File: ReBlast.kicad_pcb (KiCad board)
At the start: 2 copper layers, 50.7 x 64.9 mm, 23 parts, among them J1 MOS_8580_Socket, U1 74HC20, U2 74HC139, U3 ZN428E-8, U4 TLC272, U5 MOS_8580, U6 ADC0804

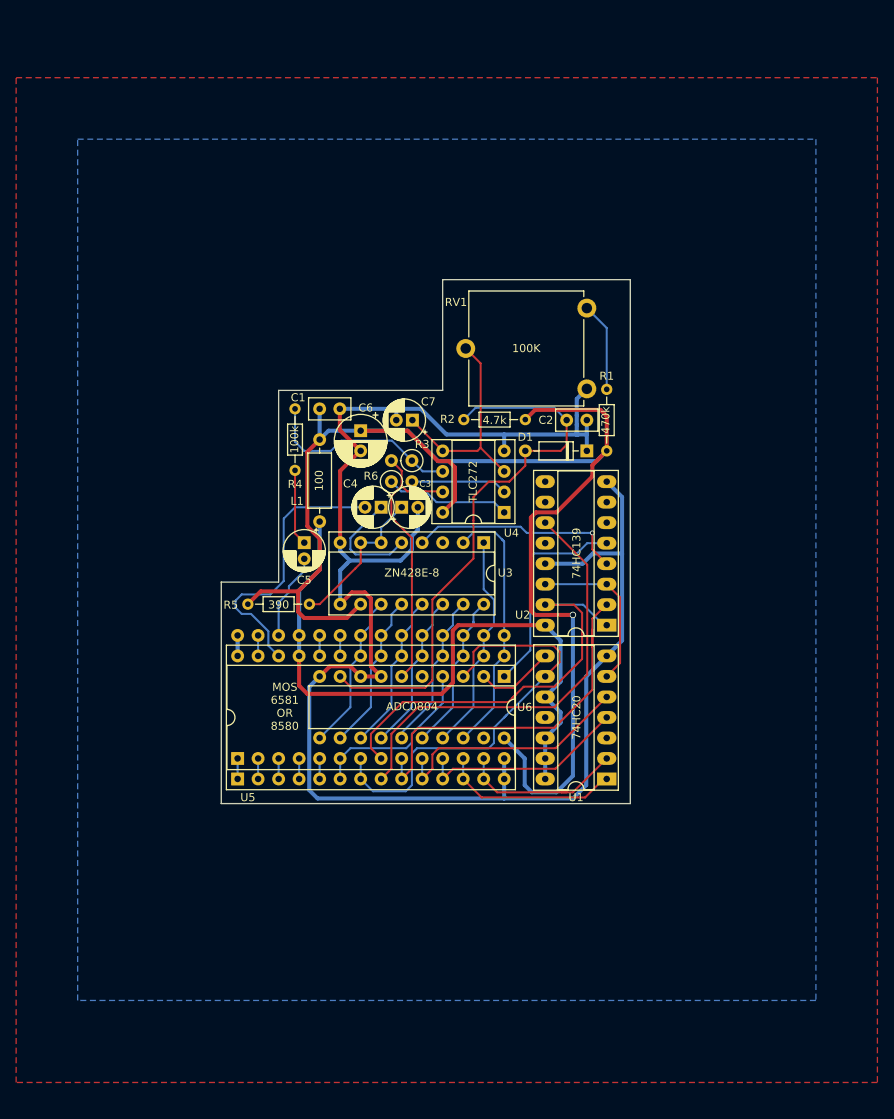
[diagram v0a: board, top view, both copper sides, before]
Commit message: Almost there...
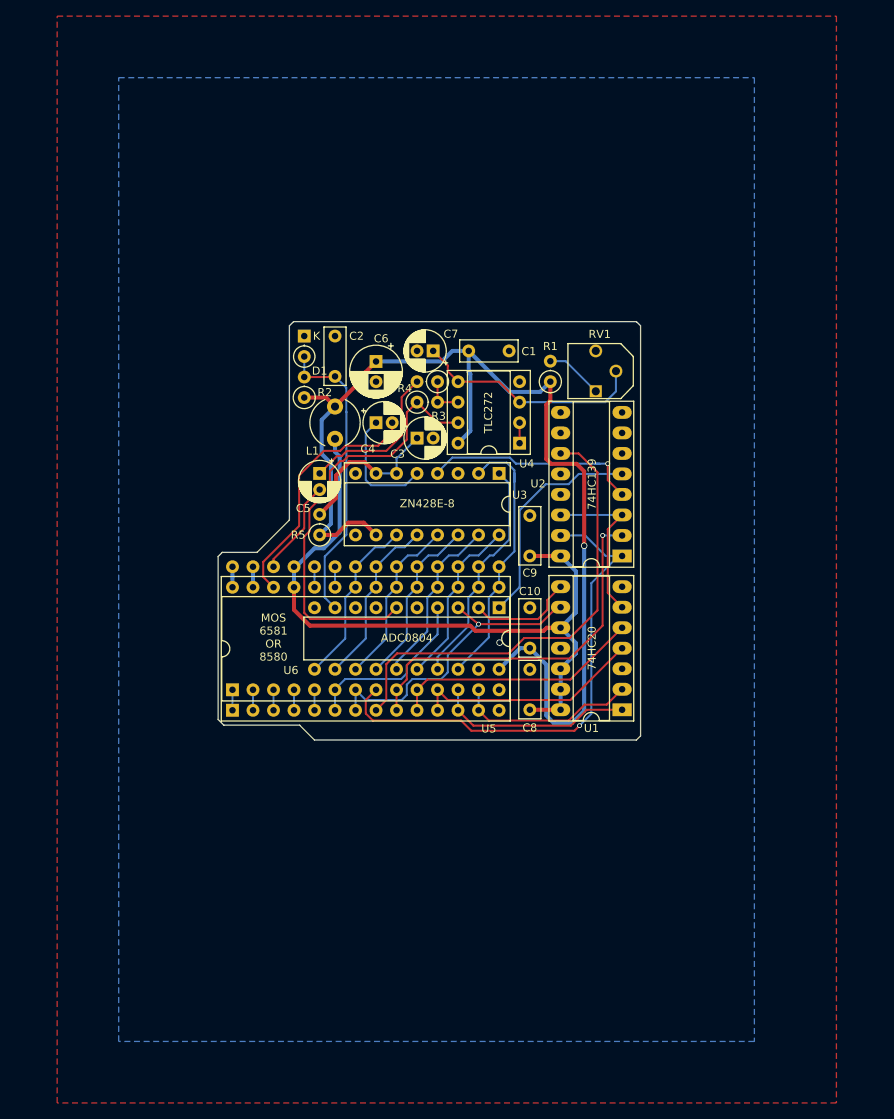
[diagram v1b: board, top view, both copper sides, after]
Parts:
- removed R6: 330k, Resistor_THT:R_Axial_DIN0207_L6.3mm_D2.5mm_P2.54mm_Vertical
- added C10: 100n, Capacitor_THT:C_Disc_D7.0mm_W2.5mm_P5.00mm, F.Cu at (165.2, 108.8)
- added C8: 100n, Capacitor_THT:C_Disc_D7.0mm_W2.5mm_P5.00mm, F.Cu at (165.2, 116.4)
- added C9: 100n, Capacitor_THT:C_Disc_D7.0mm_W2.5mm_P5.00mm, F.Cu at (165.2, 97.3)
- C1, C2: footprint Capacitor_THT:C_Disc_D5.0mm_W2.5mm_P2.50mm -> Capacitor_THT:C_Disc_D7.0mm_W2.5mm_P5.00mm
- D1: footprint Diode_THT:D_DO-35_SOD27_P7.62mm_Horizontal -> Diode_THT:D_DO-35_SOD27_P2.54mm_Vertical_KathodeUp
- L1: footprint Inductor_THT:L_Axial_L6.6mm_D2.7mm_P10.16mm_Horizontal_Vishay_IM-2 -> Inductor_THT:L_Radial_D6.0mm_P4.00mm
- R1, R2, R4, R5: footprint Resistor_THT:R_Axial_DIN0204_L3.6mm_D1.6mm_P7.62mm_Horizontal -> Resistor_THT:R_Axial_DIN0207_L6.3mm_D2.5mm_P2.54mm_Vertical
- RV1: footprint Potentiometer_THT:Potentiometer_ACP_CA14V-15_Vertical -> ReBlast:Pot_Bourns_3306P
- moved D1 37.8 mm to (137.3, 70.1), turned to 270 degrees
- moved C2 29.2 mm to (141.1, 75.1), turned to 90 degrees
- moved R2 27.5 mm to (137.3, 77.7), turned to 90 degrees
- moved C1 19.8 mm to (157.7, 71.9)
- moved R4 18.0 mm to (153.8, 75.8), turned to 180 degrees
- moved R5 12.3 mm to (139.2, 94.7), turned to 90 degrees
- moved R1 11.1 mm to (167.8, 75.8)
- moved C4 10.5 mm to (146.2, 80.8), turned to 0 degrees
- moved L1 10.4 mm to (141.1, 82.8)
- moved C7 8.95 mm to (153.3, 71.9)
- moved C3 8.78 mm to (151.3, 82.7)
- moved C5 8.78 mm to (139.2, 87.1)
- moved C6 8.78 mm to (146.2, 73.3)
- moved U1 8.78 mm to (176.7, 116.4)
- moved U2 8.78 mm to (176.7, 97.3)
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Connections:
- R3 pad 1: Net-(R3-Pad1) -> /adc_in
- R3 pad 2: /adc_in -> Net-(R3-Pad2)
- R4 pad 1: Net-(R3-Pad1) -> Net-(R3-Pad2)
- U4 pad 1: Net-(R6-Pad1) -> Net-(U4-Pad1)
- U4 pad 2: Net-(R6-Pad2) -> Net-(U4-Pad1)
- U4 pad 6: Net-(R3-Pad1) -> Net-(R3-Pad2)
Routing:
- net GNDA: track 215.1 -> 0.00 mm, vias 0 -> 1
- net +5V: track 180.9 -> 139.3 mm
- net /adc_vref_half: track 69.4 -> 37.3 mm
- net Net-(R3-Pad1): track 24.9 -> 0.00 mm
- net /adc_in: track 35.4 -> 54.1 mm
- net /r_~w: track 54.4 -> 38.5 mm, vias 0 -> 1
- net Net-(R6-Pad1): track 15.5 -> 0.00 mm
- net Net-(R6-Pad2): track 12.0 -> 0.00 mm
- net /~cs_in: track 53.5 -> 64.3 mm, vias 0 -> 1
- net Net-(C5-Pad1): track 9.43 -> 19.6 mm
- net VCC: track 81.8 -> 89.7 mm
- net Net-(R3-Pad2): track 0.00 -> 5.08 mm
- net /audio_in: track 35.1 -> 31.1 mm
- net Net-(R1-Pad2): track 11.0 -> 7.17 mm
- net /~cs_sid: track 54.4 -> 57.8 mm
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- added copper zone on B.Cu, net GNDA
- added copper zone on F.Cu, net GNDA
- removed copper zone on B.Cu, net GNDD
- removed copper zone on F.Cu, net GNDD
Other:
- board size 50.7 x 64.9 mm -> 52.3 x 51.8 mm
- board text added: "V1"
